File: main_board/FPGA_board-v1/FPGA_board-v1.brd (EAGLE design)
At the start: 171.1 x 156.7 mm, 50 parts, among them IC1 7805T, IC2 7805T, J5 XT-60BATT_LABEL, X1 22-23-2021

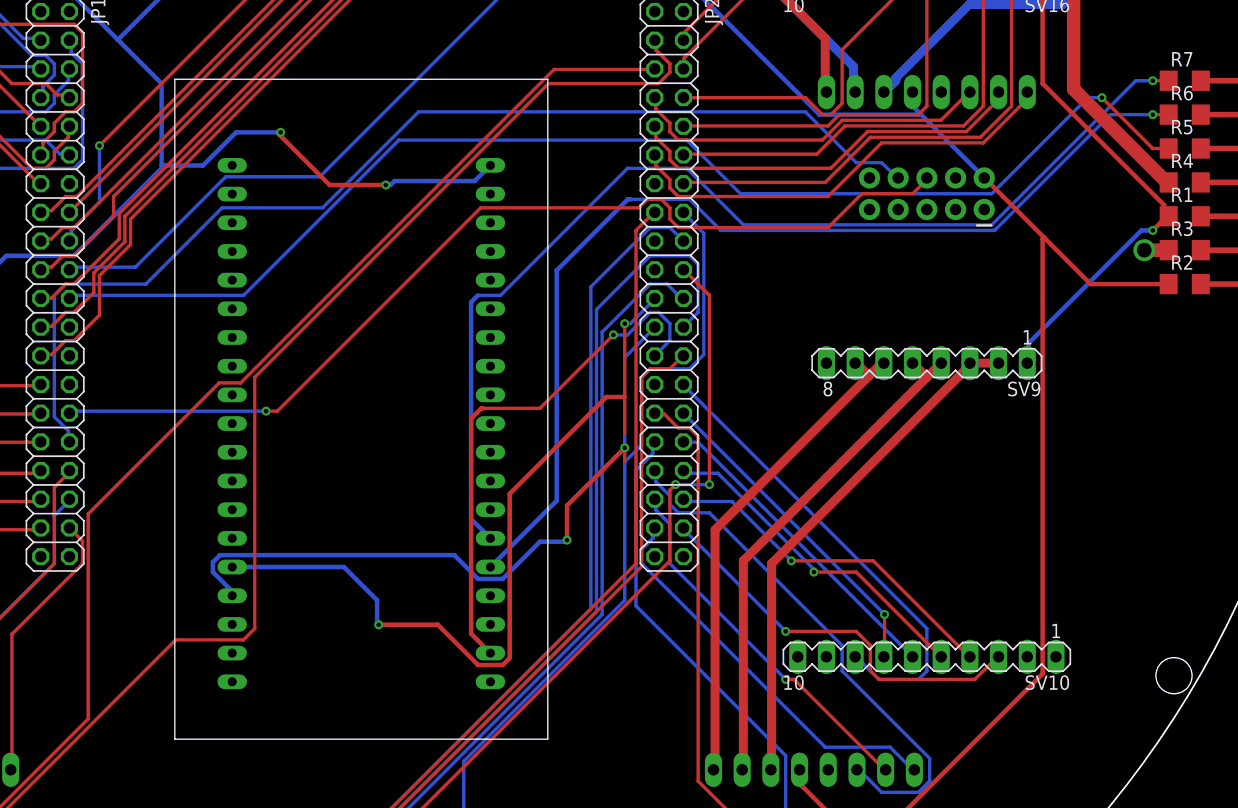
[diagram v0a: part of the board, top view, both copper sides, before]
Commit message: ESP Update
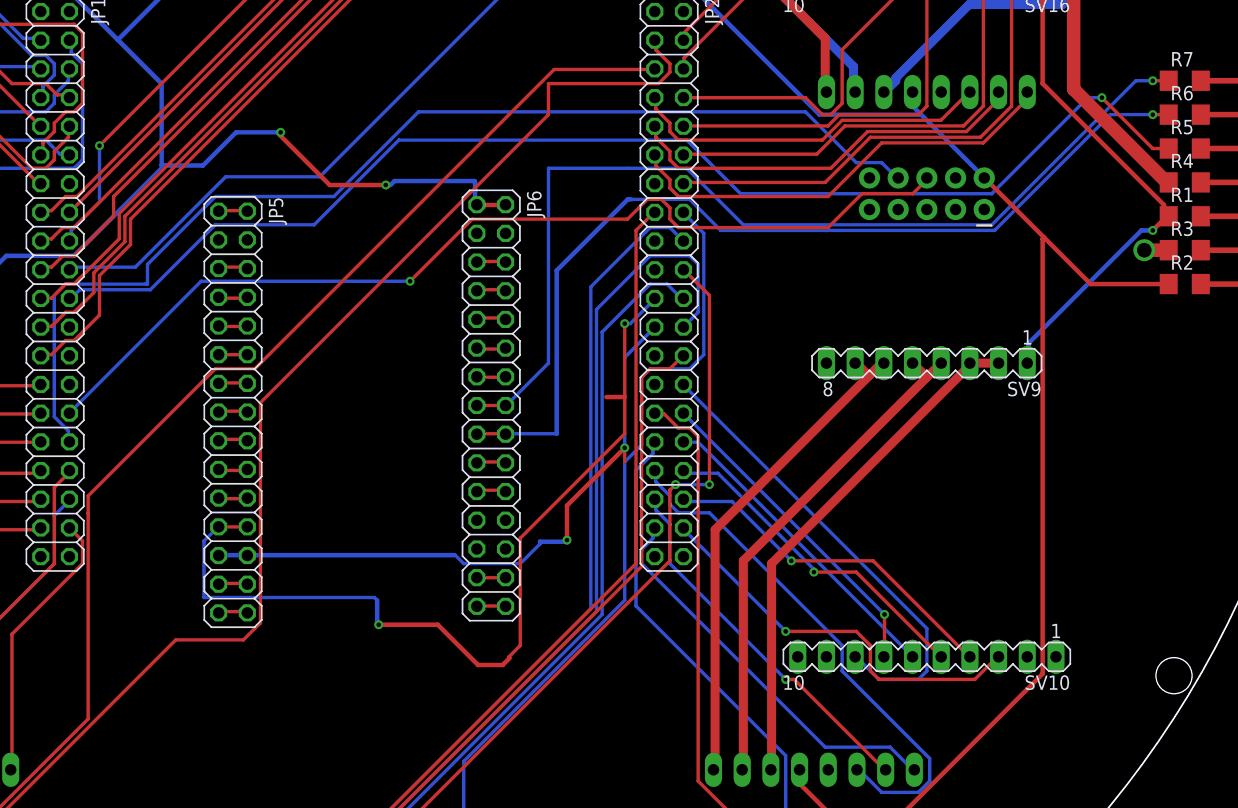
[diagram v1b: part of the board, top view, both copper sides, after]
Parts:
- removed U$1: NODEMCU32S, nodeMCU:NODEMCU32
- added JP5, JP6: (no value), pinhead:2X15
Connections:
- removed net N$2: U$1.P$17
- new net N$1: JP5.1, JP5.2
- new net N$11: JP5.11, JP5.12
- new net N$12: JP5.13, JP5.14
- new net N$14: JP5.15, JP5.16
- new net N$15: JP5.17, JP5.18
- new net N$17: JP5.19, JP5.20
- new net N$18: JP5.21, JP5.22
- new net N$23: JP5.27, JP5.28
- new net N$24: JP5.29, JP5.30
- new net N$27: JP6.5, JP6.6
- new net N$28: JP6.7, JP6.8
- new net N$29: JP6.10, JP6.9
- new net N$30: JP6.11, JP6.12
- new net N$31: JP6.13, JP6.14
- new net N$34: JP6.19, JP6.20
- new net N$35: JP6.21, JP6.22
- new net N$38: JP6.27, JP6.28
- new net N$39: JP6.29, JP6.30
- new net N$6: JP5.5, JP5.6
- new net N$8: JP5.7, JP5.8
- new net N$9: JP5.10, JP5.9
- net 5V1: now also JP6.1, JP6.2; no longer U$1.P$20
- net ESP_EN: no longer U$1.P$37
- net ESP_REC: now also JP6.15, JP6.16; no longer U$1.P$33
- net ESP_RX: now also JP5.23, JP5.24; no longer U$1.P$15
- net ESP_TRANS: now also JP6.17, JP6.18; no longer U$1.P$34
- net ESP_TX: now also JP5.25, JP5.26; no longer U$1.P$16
- net GND: now also JP5.3, JP5.4, JP6.3, JP6.4; no longer U$1.P$13, U$1.P$19, U$1.P$21, U$1.P$25
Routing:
- net ESP_EN: track 46.8 -> 0.14 mm, vias 1 -> 0
- net ESP_REC: track 95.6 -> 87.4 mm
- net ESP_RX: track 71.2 -> 79.4 mm
- net ESP_TRANS: track 91.2 -> 84.1 mm
- net ESP_TX: track 60.9 -> 55.7 mm
- net 5V1: track 299.9 -> 302.7 mm
- net N$29: track 0.00 -> 2.65 mm
- net N$6: track 0.00 -> 2.65 mm
- net N$35: track 0.00 -> 2.63 mm
- net N$15: track 0.00 -> 2.63 mm
- net N$24: track 0.00 -> 2.62 mm
- net N$28: track 0.00 -> 2.60 mm
- net N$17: track 0.00 -> 2.60 mm
- net N$8: track 0.00 -> 2.59 mm
- net N$30: track 0.00 -> 2.59 mm
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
